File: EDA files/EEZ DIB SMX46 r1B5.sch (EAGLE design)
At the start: 163 parts, among them IC1 STM32F030C6T6, IC2 74HC1G126GW,125, IC3 M24C32-WMN6P, IC4 LP2985-33DBVR, IC5 74HC2G04GW,125, IC6 OPA2990IDR, K1 FTR-C1GA012G-B05, K10 FTR-C1GA012G-B05, K11 FTR-C1GA012G-B05, K12 FTR-C1GA012G-B05, K13 FTR-C1GA012G-B05, K14 FTR-C1GA012G-B05, K15 FTR-C1GA012G-B05, K16 FTR-C1GA012G-B05, K17 FTR-C1GA012G-B05, K18 FTR-C1GA012G-B05, K19 RT424005, K2 FTR-C1GA012G-B05, K20 FTR-C1GA012G-B05, K21 FTR-C1GA012G-B05, K22 FTR-C1GA012G-B05, K23 FTR-C1GA012G-B05, K24 FTR-C1GA012G-B05, K25 FTR-C1GA012G-B05, K3 FTR-C1GA012G-B05, K4 FTR-C1GA012G-B05, K5 FTR-C1GA012G-B05, K6 FTR-C1GA012G-B05, K7 FTR-C1GA012G-B05, K8 FTR-C1GA012G-B05, K9 FTR-C1GA012G-B05, Q1 2N7002, Q10 2N7002, Q11 2N7002, Q12 2N7002, Q13 2N7002, Q14 2N7002, Q15 2N7002, Q16 2N7002, Q17 2N7002, Q18 2N7002, Q19 2N7002, Q2 2N7002, Q20 2N7002, Q21 2N7002, Q22 2N7002, Q23 2N7002, Q24 2N7002, Q25 2N7002, Q3 2N7002, Q4 2N7002, Q5 2N7002, Q6 2N7002, Q7 2N7002, Q8 2N7002, Q9 2N7002, X1 N.C., X2 77317-104-28LF, X3 691327310016, X4 691327310016, X6 DS1014-10RF1B, X7 DS1014-10RF1B

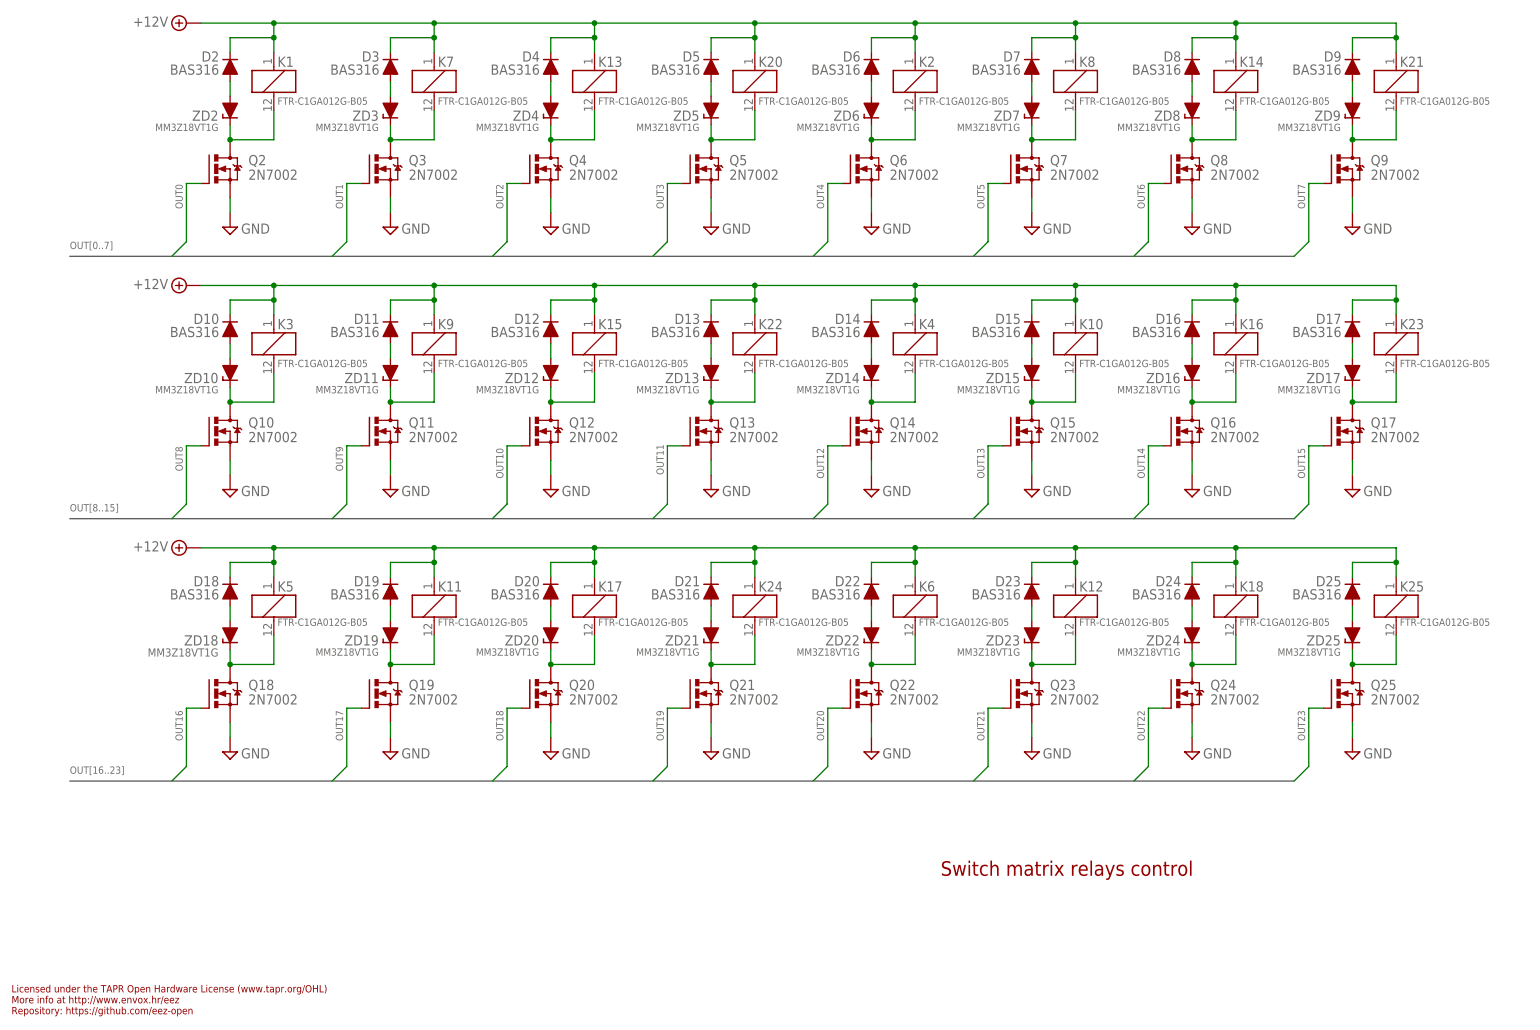
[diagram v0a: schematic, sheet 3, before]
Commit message: #5, BOM update
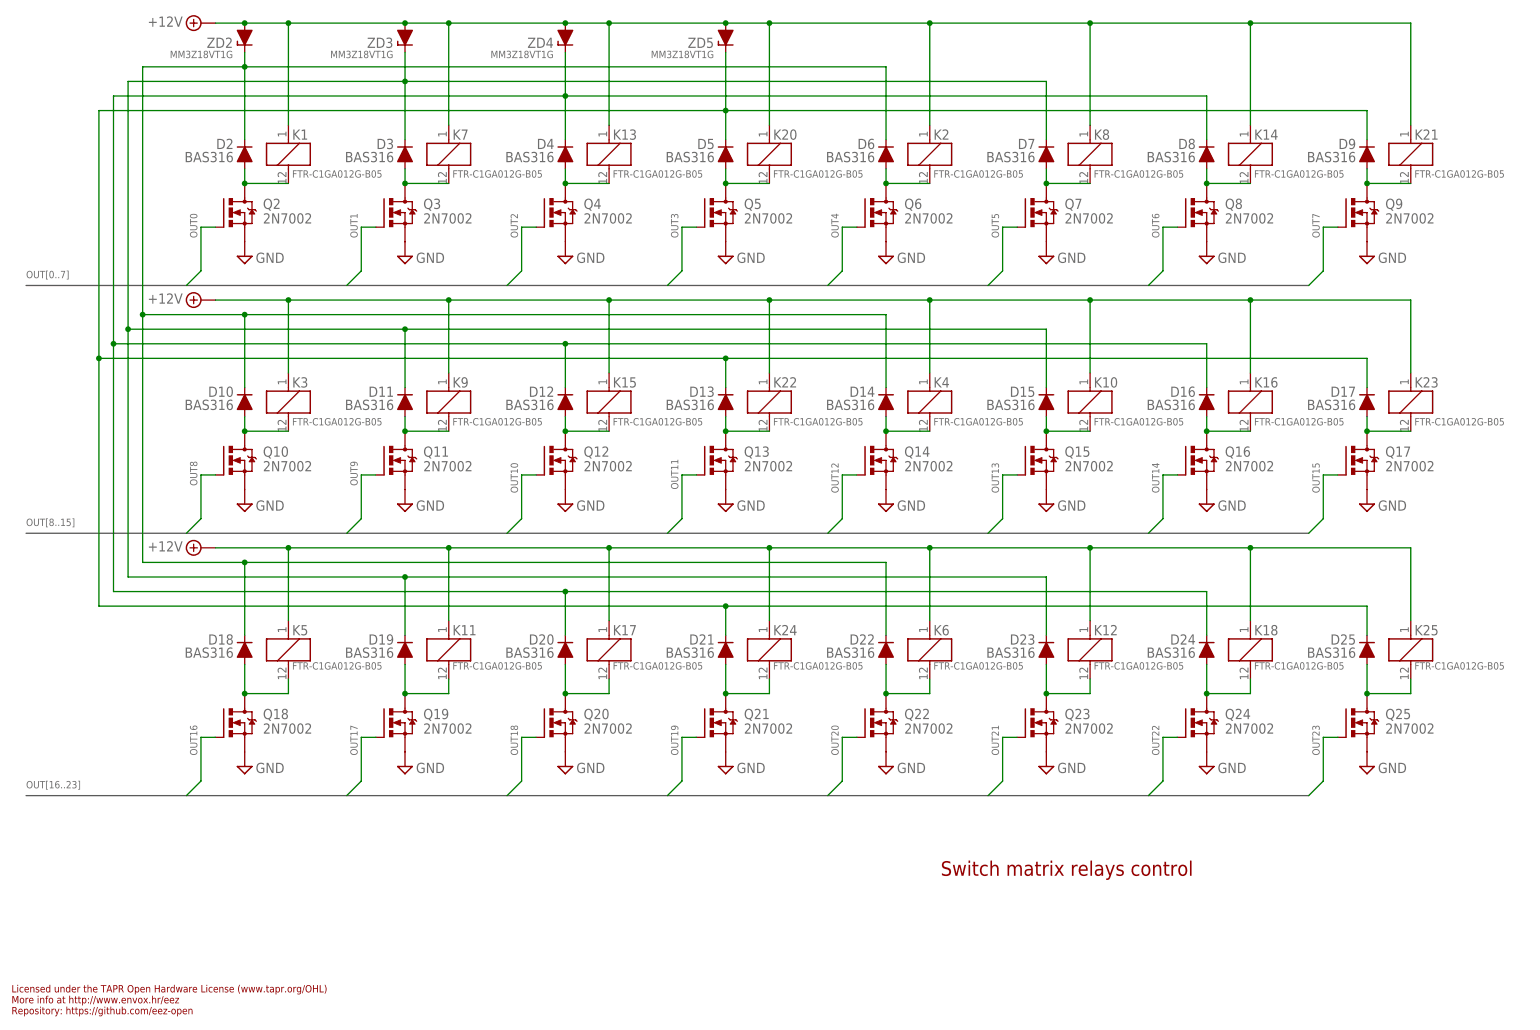
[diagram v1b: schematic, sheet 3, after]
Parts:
- removed ZD10, ZD11, ZD12, ZD13, ZD14, ZD15, ZD16, ZD17, ZD18, ZD19, ZD20, ZD21, ZD22, ZD23, ZD24, ZD25, ZD6, ZD7, ZD8, ZD9: MM3Z18VT1G, EEZ_Lib1:ZENER-DIODESOD323R
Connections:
- removed net N$13: D10.A, ZD10.A
- removed net N$18: D8.A, ZD8.A
- removed net N$22: D9.A, ZD9.A
- removed net N$26: D11.A, ZD11.A
- removed net N$28: D7.A, ZD7.A
- removed net N$30: D12.A, ZD12.A
- removed net N$32: D6.A, ZD6.A
- removed net N$36: D13.A, ZD13.A
- removed net N$38: D3.A, ZD3.A
- removed net N$40: D14.A, ZD14.A
- removed net N$42: D2.A, ZD2.A
- removed net N$44: D15.A, ZD15.A
- removed net N$46: D5.A, ZD5.A
- removed net N$48: D16.A, ZD16.A
- removed net N$50: D17.A, ZD17.A
- removed net N$52: D19.A, ZD19.A
- removed net N$54: D20.A, ZD20.A
- removed net N$56: D21.A, ZD21.A
- removed net N$58: D22.A, ZD22.A
- removed net N$60: D23.A, ZD23.A
- removed net N$62: D18.A, ZD18.A
- removed net N$64: D24.A, ZD24.A
- removed net N$66: D25.A, ZD25.A
- new net N$4: D10.C, D14.C, D18.C, D2.C, D22.C, D6.C, ZD2.C
- new net N$6: D11.C, D15.C, D19.C, D23.C, D3.C, D7.C, ZD3.C
- new net N$7: D12.C, D16.C, D20.C, D24.C, D4.C, D8.C, ZD4.C
- net +12V: now also ZD2.A, ZD3.A, ZD4.A, ZD5.A; no longer D10.C, D11.C, D12.C, D13.C, D14.C, D15.C, D16.C, D17.C, D18.C, D19.C, D2.C, D20.C, D21.C, D22.C, D23.C, D24.C, D25.C, D3.C, D4.C, D5.C, D6.C, D7.C, D8.C, D9.C
- net N$19: now also D8.A; no longer ZD8.C
- net N$21: now also D10.A; no longer ZD10.C
- net N$23: now also D9.A; no longer ZD9.C
- net N$27: now also D11.A; no longer ZD11.C
- net N$29: now also D7.A; no longer ZD7.C
- net N$31: now also D12.A; no longer ZD12.C
- net N$33: now also D6.A; no longer ZD6.C
- net N$37: now also D13.A; no longer ZD13.C
- net N$39: now also D3.A; no longer ZD3.C
- net N$41: now also D14.A; no longer ZD14.C
- net N$43: now also D2.A; no longer ZD2.C
- net N$45: now also D15.A; no longer ZD15.C
- net N$47: now also D5.A; no longer ZD5.C
- net N$49: now also D16.A; no longer ZD16.C
- net N$51: now also D17.A; no longer ZD17.C
- net N$53: now also D19.A; no longer ZD19.C
- net N$55: now also D20.A; no longer ZD20.C
- net N$57: now also D21.A; no longer ZD21.C
- net N$59: now also D22.A; no longer ZD22.C
- net N$61: now also D23.A; no longer ZD23.C
- net N$63: now also D18.A; no longer ZD18.C
- net N$65: now also D24.A; no longer ZD24.C
- net N$67: now also D25.A; no longer ZD25.C
- net N$8: now also D13.C, D17.C, D21.C, D25.C, D5.C, D9.C, ZD5.C; no longer D4.A, ZD4.A
- net N$9: now also D4.A; no longer ZD4.C
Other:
- moved on the sheet: D10, D11, D12, D13, D14, D15, D16, D17, D18, D19, D2, D20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
